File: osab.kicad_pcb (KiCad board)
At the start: 2 copper layers, 50 x 75 mm, 98 parts, among them CON1 TF-01A, CON2 PJ-3420-A-SMT, CON3 TYPE-C-31-M-12, Q1 BC847B, Q2 BC847B, SW1 PPP, SW10 RESET, SW11 Torch, SW2 VOL-, SW3 VOL+, SW4 CHAP-, SW5 CHAP+, SW6 OT/NT, SW7 BOOK-, SW8 BOOK+, SW9 XKB5858-Z-F, U1 VS1000, U2 ME6211C33M5G-N, U3 CAT25640, U4 TP4055, U5 MF5853CS, U6 PAM8302AAS, Y1 12MHz

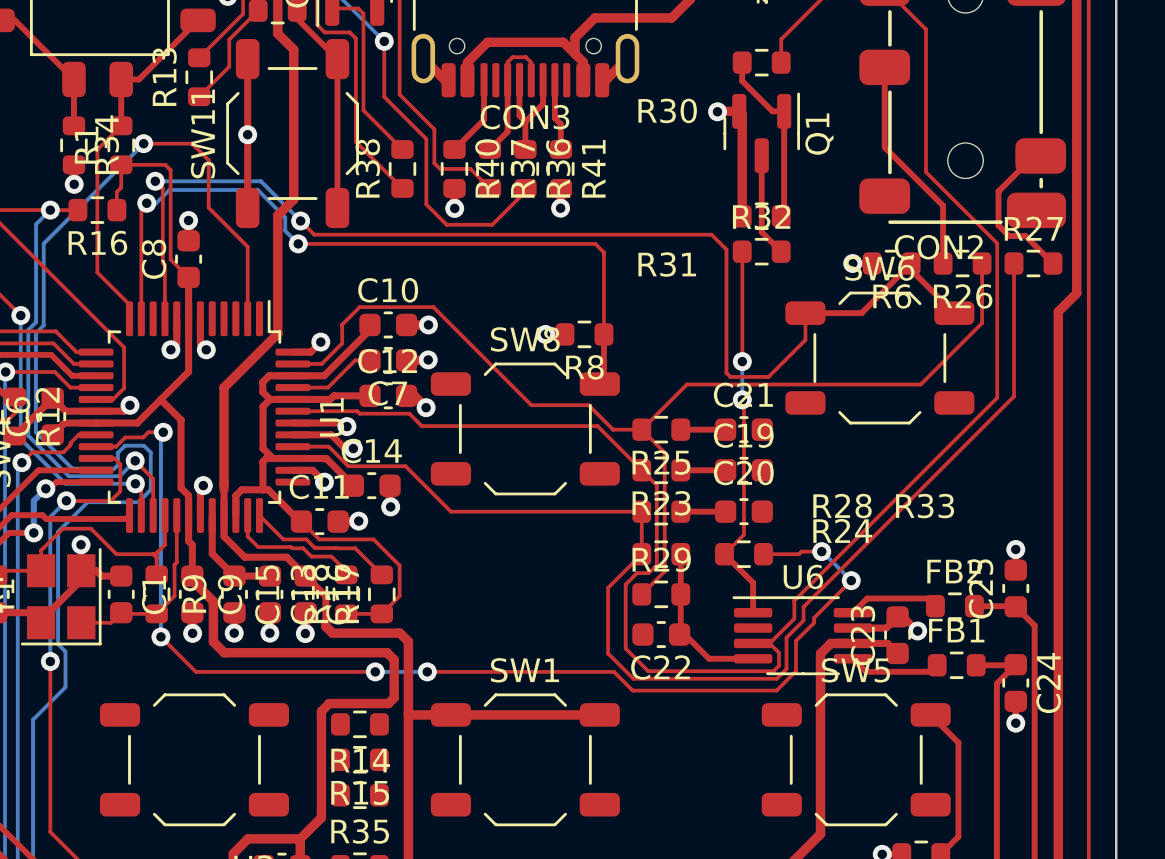
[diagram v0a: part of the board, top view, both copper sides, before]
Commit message: production: Routing tracks...
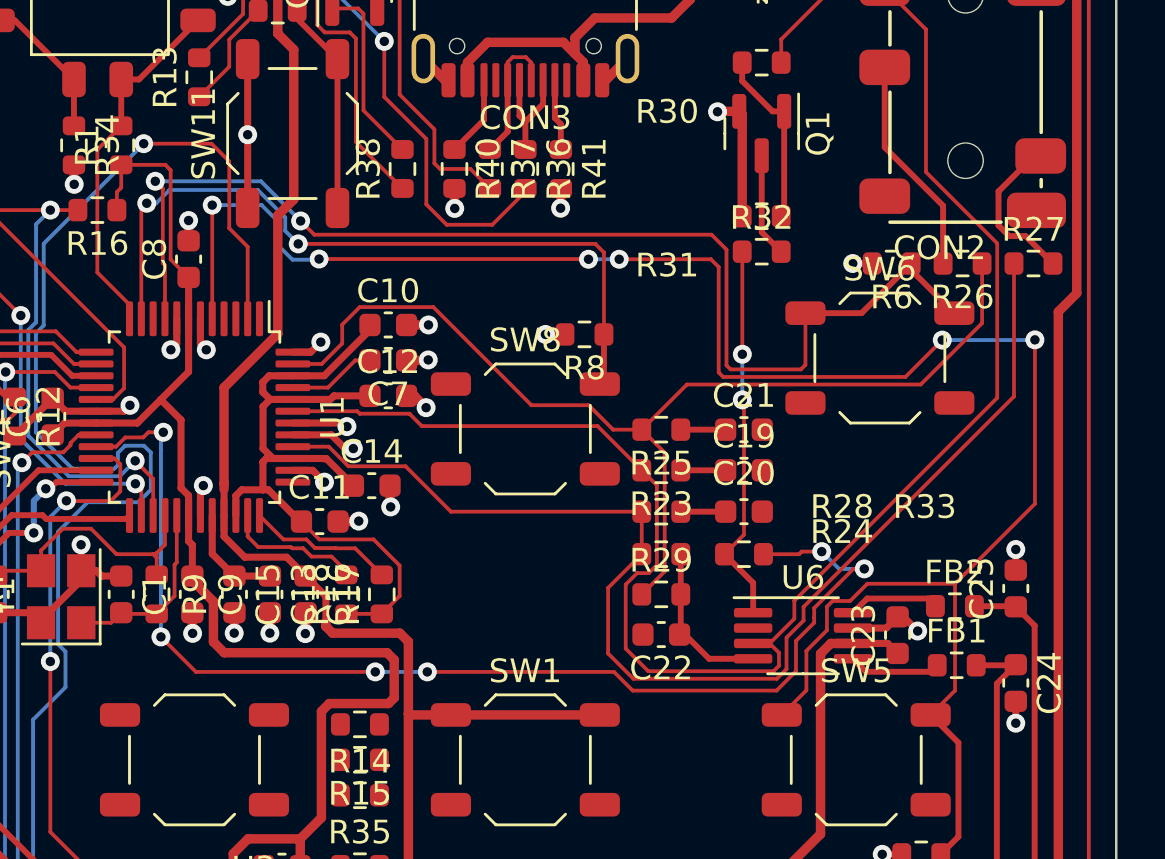
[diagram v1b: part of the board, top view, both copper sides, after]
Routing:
- net Net-(R5-Pad1): track 6.70 -> 82.1 mm, vias 0 -> 6
- net Net-(R33-Pad2): track 49.0 -> 50.4 mm
